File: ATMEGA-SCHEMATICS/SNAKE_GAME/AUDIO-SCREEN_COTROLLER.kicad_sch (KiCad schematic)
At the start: 40 parts, among them J19 PCF_SCREEN, SW3 SWS_Push, U3 PCF8574AP, Y3 Crystal

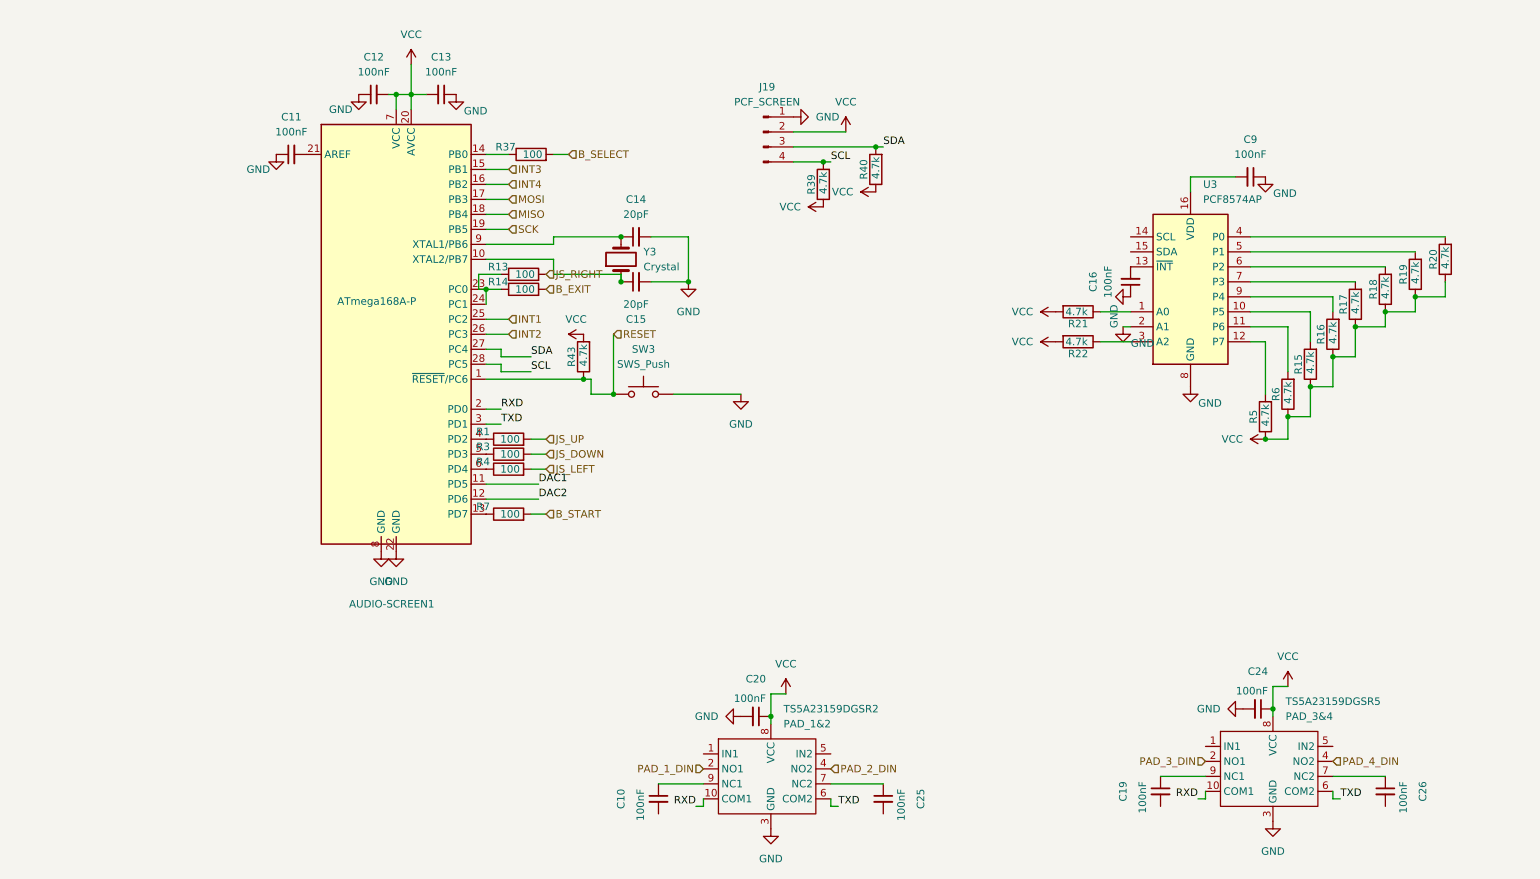
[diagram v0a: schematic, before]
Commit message: .
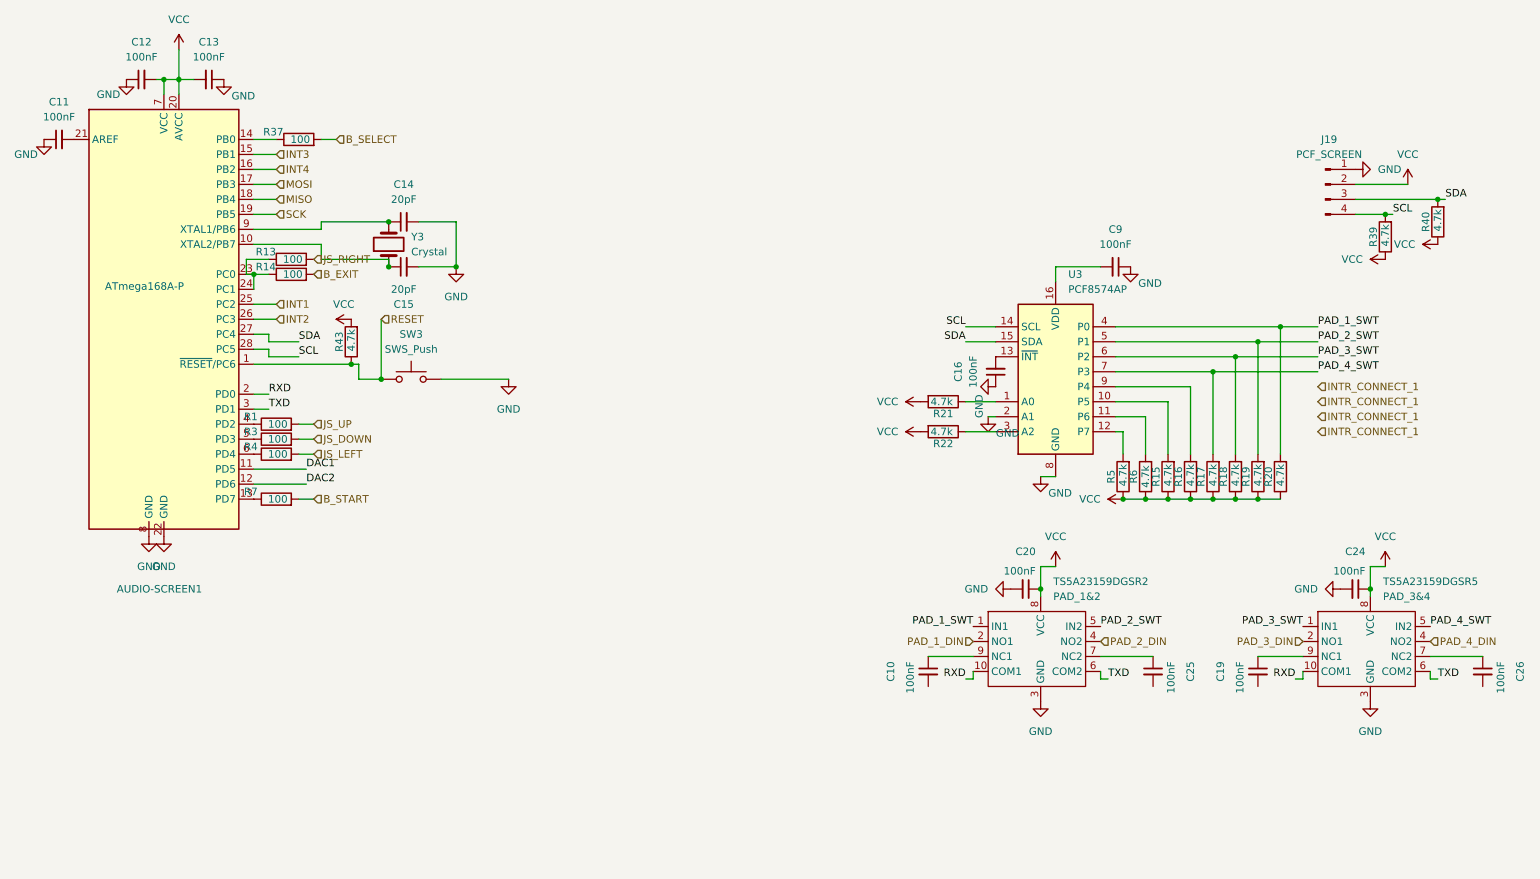
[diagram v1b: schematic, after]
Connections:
- net SCL: now also U3.14 (SCL)
- net SDA: now also U3.15 (SDA)
- net PAD_2_SWT: now reaches R19.2, U3.5 (P1)
- net PAD_2_SWT: now also TS5A23159DGSR2.5 (IN2)
- net PAD_4_SWT: now reaches R17.2, U3.7 (P3)
- net PAD_4_SWT: now also TS5A23159DGSR5.5 (IN2)
- net PAD_3_SWT: now reaches R18.2, U3.6 (P2)
- net PAD_3_SWT: now also TS5A23159DGSR5.1 (IN1)
- net PAD_1_SWT: now reaches TS5A23159DGSR2.1 (IN1)
- net PAD_1_SWT: now also R20.2, U3.4 (P0)
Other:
- moved on the sheet: AUDIO-SCREEN1, C10, C11, C12, C13, C14, C15, C16, C19, C20, C24, C25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
